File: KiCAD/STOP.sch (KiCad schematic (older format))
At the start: 64 parts

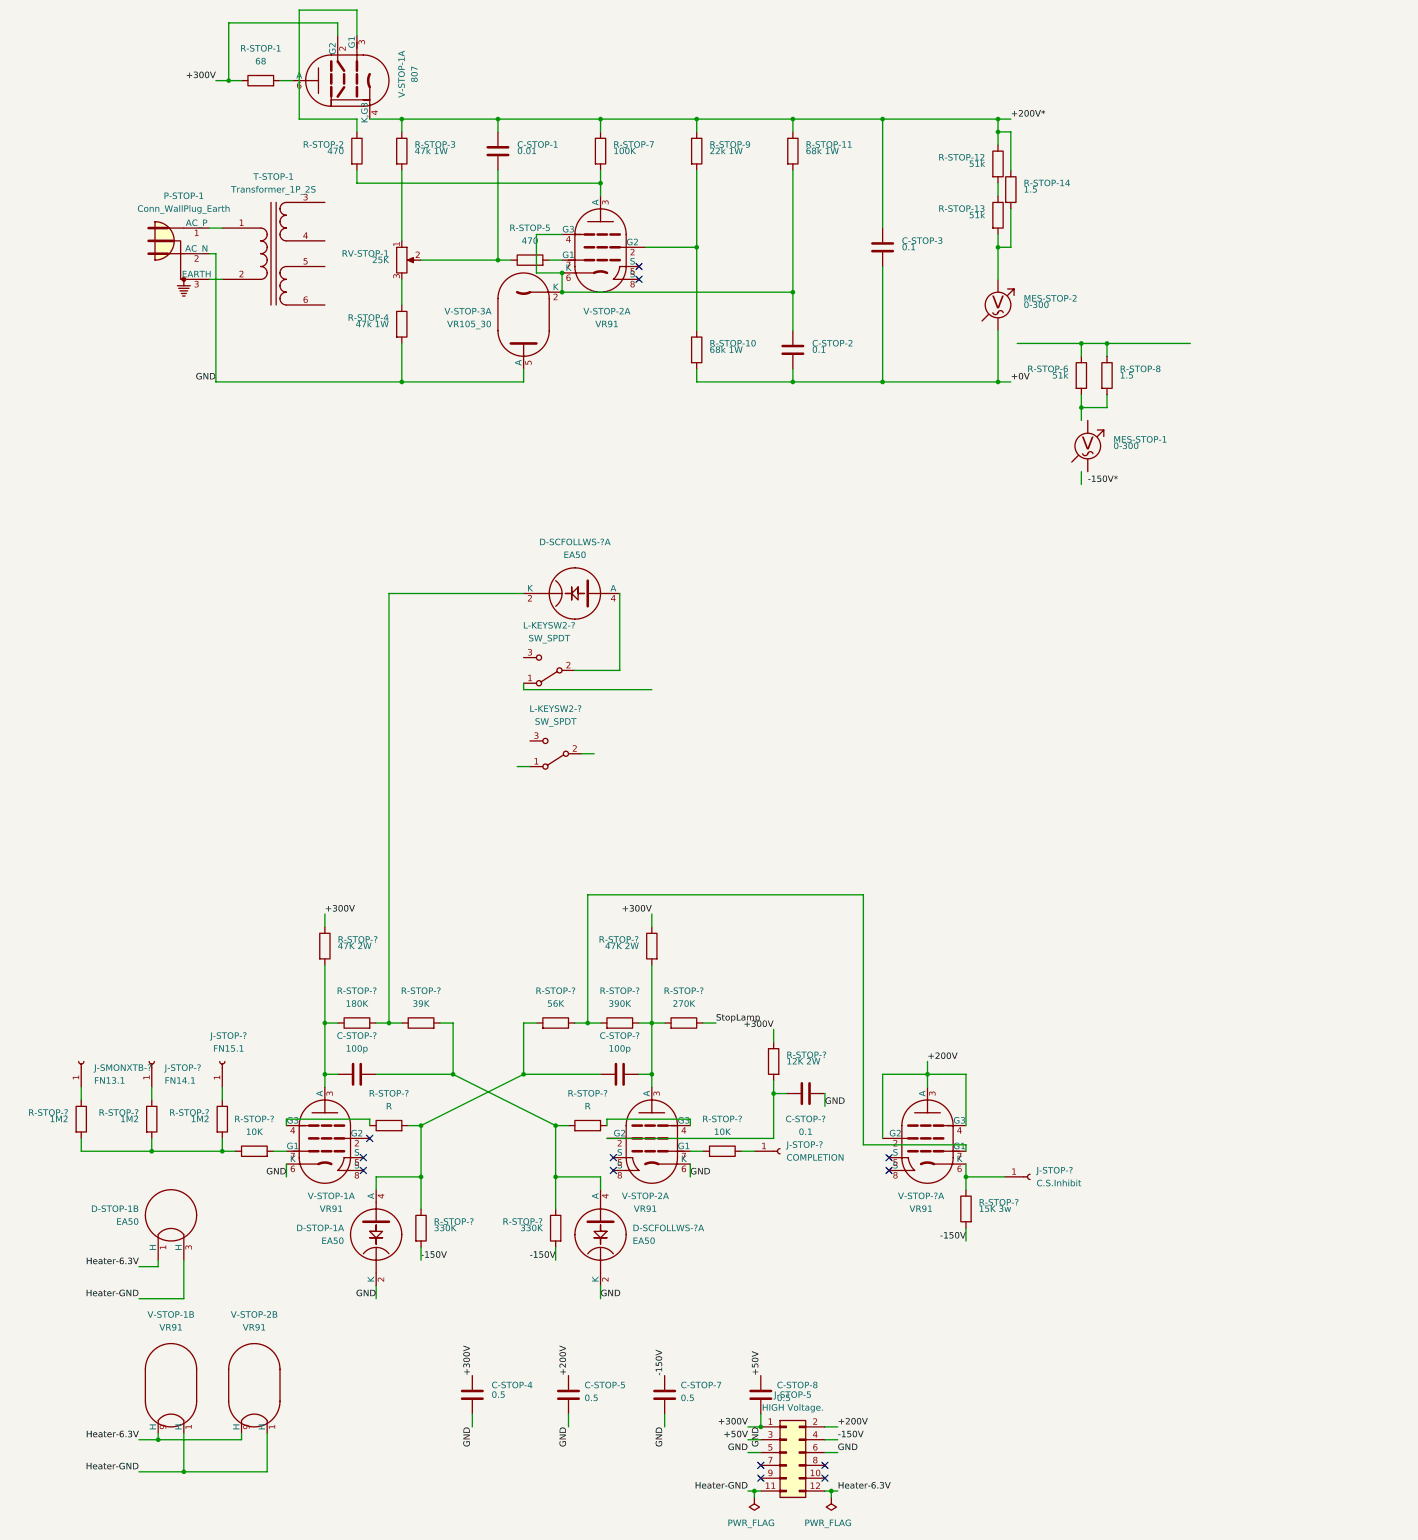
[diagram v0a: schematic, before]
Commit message: Add StorGate & some Valve Logic data.
Signed-off-by: John Bradley <flypie@rocketmail.com>
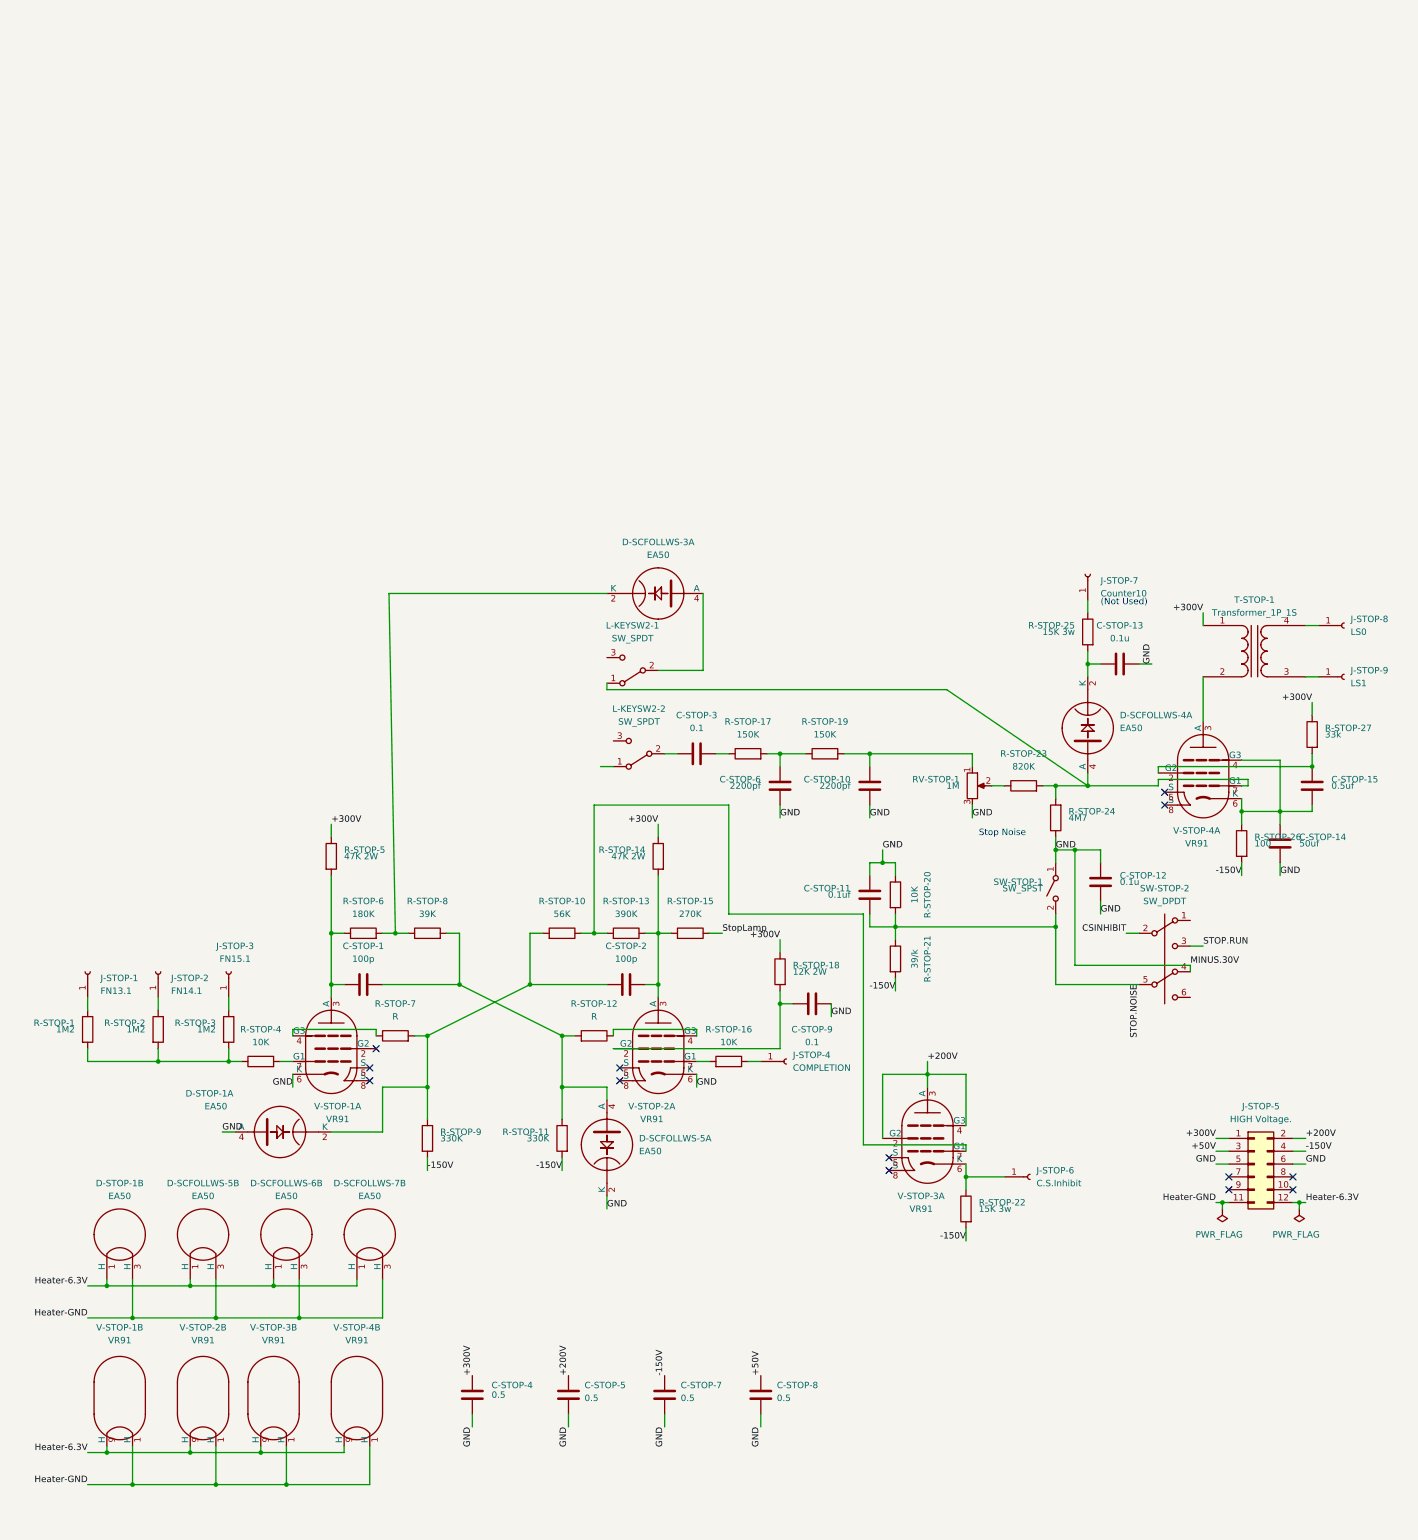
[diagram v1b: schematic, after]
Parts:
- removed C-STOP-1: 0.01, Capacitor_THT:C_Disc_D7.5mm_W5.0mm_P5.00mm, symbol Device:C
- removed C-STOP-?: 100p, Capacitor_THT:C_Disc_D7.5mm_W5.0mm_P5.00mm, symbol Device:C
- removed D-SCFOLLWS-?: EA50, NewValves:Valve_B3G, symbol NEWValves:EA50
- removed J-STOP-?: FN14.1, SamacSys_Parts_l:242431, symbol Connector:Conn_01x01_Female
- removed J-STOP-?: COMPLETION, SamacSys_Parts_l:242431, symbol Connector:Conn_01x01_Female
- removed J-STOP-?: C.S.Inhibit, SamacSys_Parts_l:242431, symbol Connector:Conn_01x01_Female
- removed L-KEYSW2-? (x2): SW_SPDT, SamacSys_Parts_m:A101SYCQ04, symbol Switch:SW_SPDT
- removed MES-STOP-1, MES-STOP-2: 0-300, Connector_PinSocket_2.54mm:PinSocket_1x02_P2.54mm_Vertical, symbol Device:Voltmeter_AC
- removed P-STOP-1: Conn_WallPlug_Earth, Connector_PinSocket_2.54mm:PinSocket_1x03_P2.54mm_Vertical, symbol Connector:Conn_WallPlug_Earth
- removed R-STOP-14, R-STOP-8: 1.5, Resistor_THT:R_Axial_DIN0516_L15.5mm_D5.0mm_P5.08mm_Vertical, symbol Device:R
- removed R-STOP-5: 470, Resistor_THT:R_Axial_DIN0516_L15.5mm_D5.0mm_P5.08mm_Vertical, symbol Device:R
- removed R-STOP-6: 51k, Resistor_THT:R_Axial_DIN0516_L15.5mm_D5.0mm_P5.08mm_Vertical, symbol Device:R
- removed R-STOP-7: 100K, Resistor_THT:R_Axial_DIN0516_L15.5mm_D5.0mm_P5.08mm_Vertical, symbol Device:R
- removed R-STOP-? (x2): 10K, Resistor_THT:R_Axial_DIN0516_L15.5mm_D5.0mm_P5.08mm_Vertical, symbol Device:R
- removed R-STOP-? (x3): 1M2, Resistor_THT:R_Axial_DIN0516_L15.5mm_D5.0mm_P5.08mm_Vertical, symbol Device:R
- removed R-STOP-? (x2): 330K, Resistor_THT:R_Axial_DIN0516_L15.5mm_D5.0mm_P5.08mm_Vertical, symbol Device:R
- removed R-STOP-?: R, Resistor_THT:R_Axial_DIN0516_L15.5mm_D5.0mm_P5.08mm_Vertical, symbol Device:R
- removed R-STOP-?: 390K, Resistor_THT:R_Axial_DIN0516_L15.5mm_D5.0mm_P5.08mm_Vertical, symbol Device:R
- removed R-STOP-?: 56K, Resistor_THT:R_Axial_DIN0516_L15.5mm_D5.0mm_P5.08mm_Vertical, symbol Device:R
- removed R-STOP-?: 270K, Resistor_THT:R_Axial_DIN0516_L15.5mm_D5.0mm_P5.08mm_Vertical, symbol Device:R
- removed R-STOP-?: 15K 3w, Resistor_THT:R_Axial_DIN0516_L15.5mm_D5.0mm_P5.08mm_Vertical, symbol Device:R
- removed T-STOP-1: Transformer_1P_2S, Connector_PinSocket_2.54mm:PinSocket_1x06_P2.54mm_Vertical, symbol Device:Transformer_1P_2S
- removed V-STOP-1: 807, NewValves:USM5+1, symbol NEWValves:807
- removed V-STOP-2: VR91, NewValves:Valve_9Loctal, symbol NEWValves:VR91
- removed V-STOP-3: VR105_30, Valve:Valve_Octal, symbol NEWValves:VR105_30
- added C-STOP-10, C-STOP-6: 2200pf, Capacitor_THT:C_Disc_D7.5mm_W5.0mm_P5.00mm, symbol Device:C
- added C-STOP-11: 0.1uf, Capacitor_THT:C_Disc_D7.5mm_W5.0mm_P5.00mm, symbol Device:C
- added C-STOP-12, C-STOP-13: 0.1u, Capacitor_THT:C_Disc_D7.5mm_W5.0mm_P5.00mm, symbol Device:C
- added C-STOP-14: 50uf, Capacitor_THT:C_Disc_D7.5mm_W5.0mm_P5.00mm, symbol Device:C
- added C-STOP-15: 0.5uf, Capacitor_THT:C_Disc_D7.5mm_W5.0mm_P5.00mm, symbol Device:C
- added D-SCFOLLWS-3, D-SCFOLLWS-4, D-SCFOLLWS-6, D-SCFOLLWS-7: EA50, NewValves:Valve_B3G, symbol NEWValves:EA50
- added unit 2 of D-SCFOLLWS-5
- added J-STOP-2: FN14.1, SamacSys_Parts_l:242431, symbol Connector:Conn_01x01_Female
- added J-STOP-4: COMPLETION, SamacSys_Parts_l:242431, symbol Connector:Conn_01x01_Female
- added J-STOP-6: C.S.Inhibit, SamacSys_Parts_l:242431, symbol Connector:Conn_01x01_Female
- added J-STOP-7: Counter10, SamacSys_Parts_l:242431, symbol Connector:Conn_01x01_Female
- added J-STOP-8: LS0, SamacSys_Parts_l:242431, symbol Connector:Conn_01x01_Female
- added J-STOP-9: LS1, SamacSys_Parts_l:242431, symbol Connector:Conn_01x01_Female
- added L-KEYSW2-1, L-KEYSW2-2: SW_SPDT, SamacSys_Parts_m:A101SYCQ04, symbol Switch:SW_SPDT
- added R-STOP-15: 270K, Resistor_THT:R_Axial_DIN0516_L15.5mm_D5.0mm_P5.08mm_Vertical, symbol Device:R
- added R-STOP-16, R-STOP-20: 10K, Resistor_THT:R_Axial_DIN0516_L15.5mm_D5.0mm_P5.08mm_Vertical, symbol Device:R
- added R-STOP-17, R-STOP-19: 150K, Resistor_THT:R_Axial_DIN0516_L15.5mm_D5.0mm_P5.08mm_Vertical, symbol Device:R
- added R-STOP-21: 39/k, Resistor_THT:R_Axial_DIN0516_L15.5mm_D5.0mm_P5.08mm_Vertical, symbol Device:R
- added R-STOP-22, R-STOP-25: 15K 3w, Resistor_THT:R_Axial_DIN0516_L15.5mm_D5.0mm_P5.08mm_Vertical, symbol Device:R
- added R-STOP-23: 820K, Resistor_THT:R_Axial_DIN0516_L15.5mm_D5.0mm_P5.08mm_Vertical, symbol Device:R
- added R-STOP-24: 4M7, Resistor_THT:R_Axial_DIN0516_L15.5mm_D5.0mm_P5.08mm_Vertical, symbol Device:R
- added R-STOP-26: 100, Resistor_THT:R_Axial_DIN0516_L15.5mm_D5.0mm_P5.08mm_Vertical, symbol Device:R
- added R-STOP-27: 33k, Resistor_THT:R_Axial_DIN0516_L15.5mm_D5.0mm_P5.08mm_Vertical, symbol Device:R
- added SW-STOP-1: SW_SPST, Connector_PinHeader_2.54mm:PinHeader_1x03_P2.54mm_Vertical, symbol Switch:SW_SPST
- added SW-STOP-2: SW_DPDT, Connector_PinHeader_2.54mm:PinHeader_1x06_P2.54mm_Vertical, symbol NEWValves:SW_DPDT
- added T-STOP-1: Transformer_1P_1S, Connector_PinHeader_2.54mm:PinHeader_1x04_P2.54mm_Vertical, symbol Device:Transformer_1P_1S
- added unit 2 of V-STOP-3
- added V-STOP-4: VR91, NewValves:Valve_9Loctal, symbol NEWValves:VR91
- C-STOP-2: value 0.1 -> 100p
- R-STOP-1: value 68 -> 1M2
- R-STOP-10: value 68k 1W -> 56K
- R-STOP-11: value 68k 1W -> 330K
- R-STOP-12: value 51k -> R
- R-STOP-13: value 51k -> 390K
- R-STOP-2: value 470 -> 1M2
- R-STOP-3: value 47k 1W -> 1M2
- R-STOP-4: value 47k 1W -> 10K
- R-STOP-9: value 22k 1W -> 330K
- RV-STOP-1: value 25K -> 1M
- gave numbers to parts that had none: 12
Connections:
- net labels added: CSINHIBIT, MINUS.30V, STOP.NOISE, STOP.RUN
- net labels removed: +0V, +200V*, -150V*
- wire segments 197 -> 210
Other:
- note added: "(Not Used)"
- note added: "Stop Noise"
- moved on the sheet: C-STOP-1, C-STOP-9, D-SCFOLLWS-5A, J-STOP-1, J-STOP-3, R-STOP-14, R-STOP-18, R-STOP-5, R-STOP-6, R-STOP-7, R-STOP-8, V-STOP-1A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
